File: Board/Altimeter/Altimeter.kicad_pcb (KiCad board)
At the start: 2 copper layers, 40 x 40 mm, 53 parts, among them J1 PWRIN, J2 STLink, J3 Micro_SD_Card_Det_Hirose_DM3AT, J4 GNSS, J5 RS485, J6 ReleaseSys, SW1 SW_RESET, U1 STM32L431RBTx, U2 LPS22HB_Module, U3 ST1480AxDR, Y1 FA238-20MHz, Y2 FC255-32.768kHz

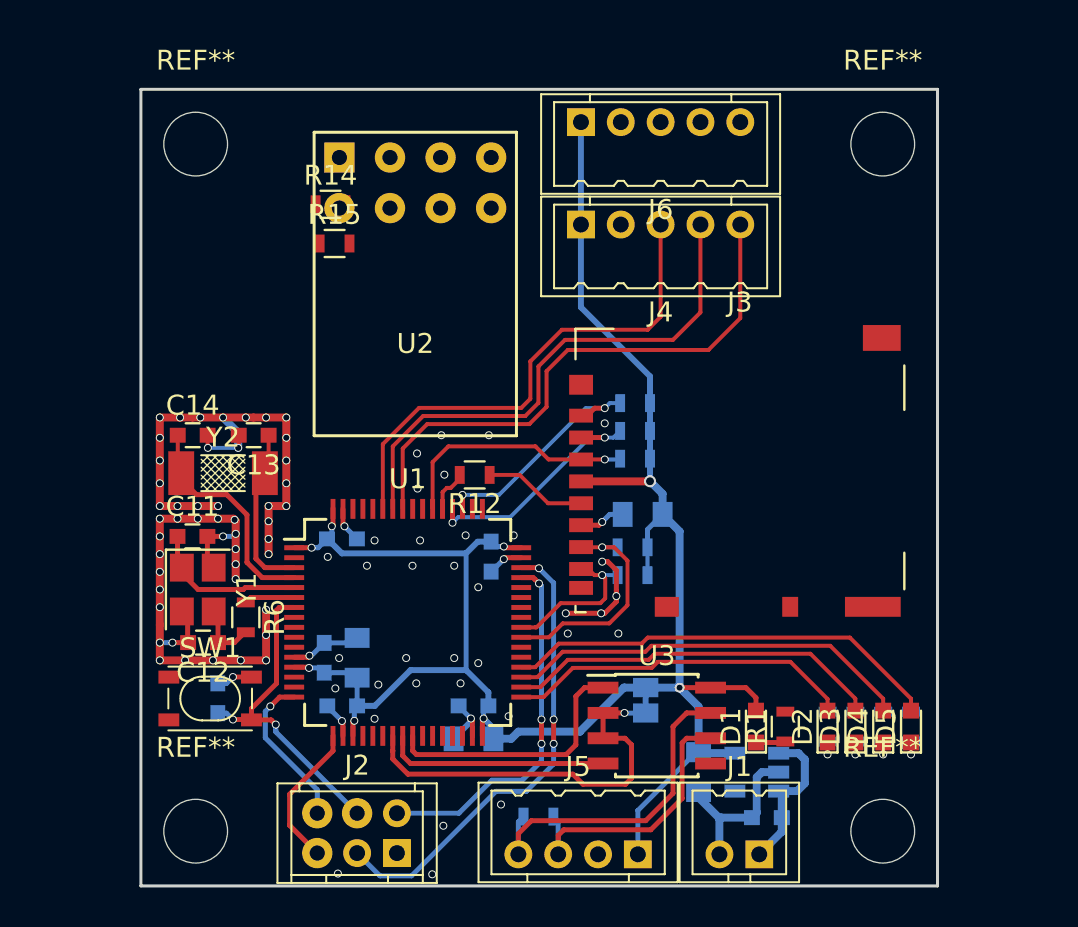
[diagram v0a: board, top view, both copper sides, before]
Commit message: almost complete (size:50x30) task: silk and via
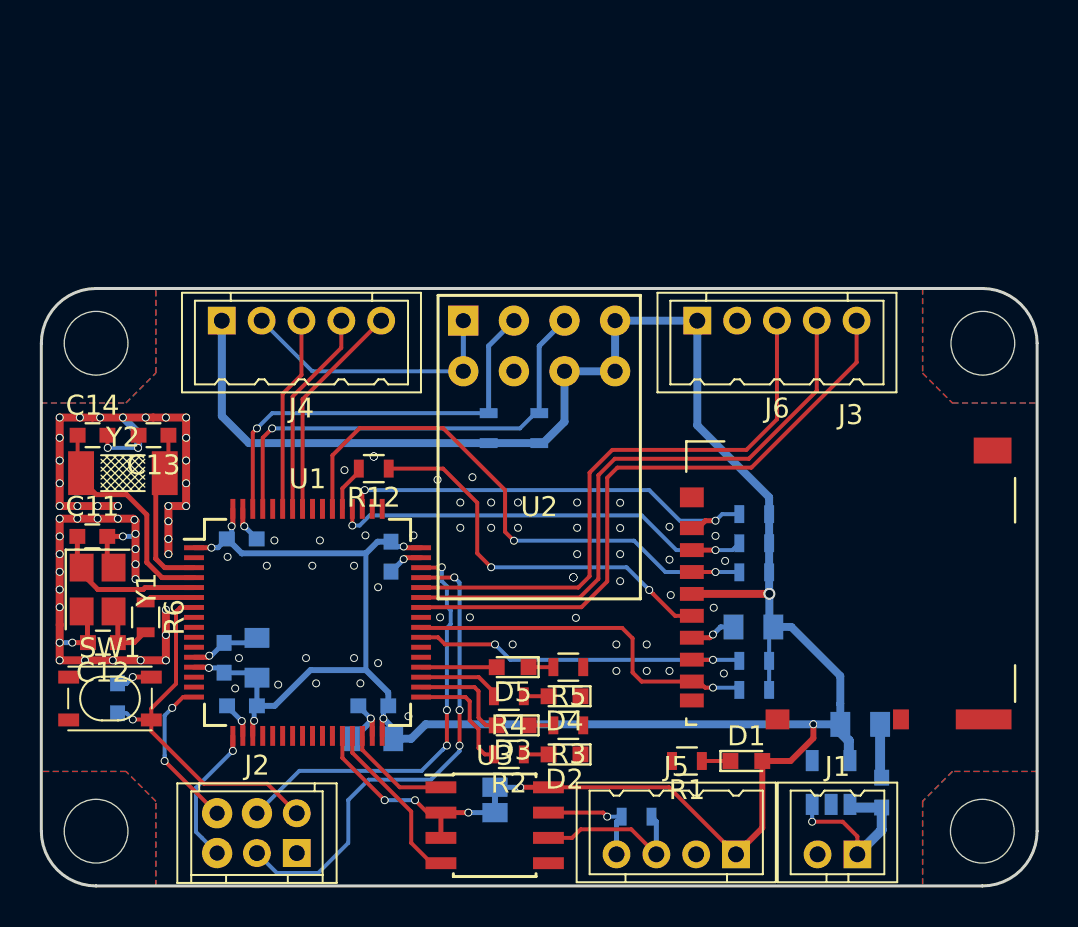
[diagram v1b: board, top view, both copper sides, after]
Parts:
- removed the REF** at (167.2, 62.8)
- removed the REF** at (167.2, 97.2)
- removed the REF** at (132.8, 97.2)
- added REF**: MountingHole_3.2mm_M3, Mounting_Holes:MountingHole_3.2mm_M3, F.Cu at (172.3, 72.8)
- added REF**: MountingHole_3.2mm_M3, Mounting_Holes:MountingHole_3.2mm_M3, F.Cu at (172.2, 97.2)
- added REF**: MountingHole_3.2mm_M3, Mounting_Holes:MountingHole_3.2mm_M3, F.Cu at (127.8, 97.2)
- R14, R15: moved to B.Cu
- R2, R3, R4, R5: moved to F.Cu
- moved D5 20.2 mm to (148.7, 89.0), turned to 180 degrees
- moved R4 18.9 mm to (148.5, 90.5), turned to 180 degrees
- moved J4 18.7 mm to (138.1, 71.6)
- moved R5 17.5 mm to (151.5, 89.0), turned to 180 degrees
- moved D3 17.2 mm to (148.7, 91.9), turned to 180 degrees
- moved D4 16.1 mm to (151.3, 90.5), turned to 180 degrees
- moved R2 16.1 mm to (148.5, 93.4), turned to 180 degrees
- moved R3 14.4 mm to (151.5, 91.9), turned to 180 degrees
- moved R15 13.8 mm to (150.0, 77.0), turned to 90 degrees
- moved R14 13.8 mm to (147.5, 77.0), turned to 90 degrees
- moved D2 13.3 mm to (151.3, 93.4), turned to 180 degrees
- moved J6 11.6 mm to (161.9, 71.6)
- moved REF** 11.2 mm to (127.8, 72.8)
- moved U2 10.3 mm to (150.0, 78.0)
- moved U3 9.56 mm to (147.8, 97.0)
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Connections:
- D2 pad 1: Net-(D2-Pad1) -> GND
- D2 pad 2: /LED_R -> Net-(D2-Pad2)
- D4 pad 1: Net-(D4-Pad1) -> GND
- D4 pad 2: /LED_G -> Net-(D4-Pad2)
- J2 pad 2: /SWDIO -> /RESET
- J2 pad 3: /SWCLK -> /SWDIO
- J2 pad 4: /RESET -> /SWCLK
- J6 pad 3: (no net) -> /TRIGGER
- J6 pad 4: (no net) -> /BUZZER
- J6 pad 5: (no net) -> /FLIGHTPIN
- R2 pad 1: GND -> Net-(D2-Pad2)
- R2 pad 2: Net-(D2-Pad1) -> /LED_R
- R4 pad 1: GND -> Net-(D4-Pad2)
- R4 pad 2: Net-(D4-Pad1) -> /LED_G
- U1 pad 23: /RS485_EN -> (no net)
- U1 pad 24: /RS485_TX -> (no net)
- U1 pad 25: /RS485_RX -> (no net)
- U1 pad 28: (no net) -> /RS485_EN
- U1 pad 29: (no net) -> /RS485_TX
- U1 pad 30: (no net) -> /RS485_RX
- U1 pad 42: (no net) -> /FLIGHTPIN
- U1 pad 43: (no net) -> /BUZZER
- U1 pad 44: (no net) -> /TRIGGER
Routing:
- net +3V3: track 101.7 -> 150.2 mm, vias 8 -> 9
- net /FLIGHTPIN: track 0.00 -> 32.1 mm
- net /BUZZER: track 0.00 -> 30.7 mm
- net /TRIGGER: track 0.00 -> 29.4 mm
- net /I2C1_SCL: track 0.00 -> 23.1 mm, vias 0 -> 1
- net /I2C1_SDA: track 0.00 -> 21.3 mm, vias 0 -> 1
- net /LED_B: track 22.1 -> 3.80 mm
- net /GNSS_1PPS: track 28.4 -> 11.1 mm
- net /SD_CMD: track 12.4 -> 29.1 mm, vias 1 -> 2
- net /GNSS_TX: track 26.9 -> 10.5 mm
- net /LED_G: track 20.5 -> 4.17 mm
- net /GNSS_RX: track 25.6 -> 9.84 mm
- net Net-(J3-Pad5): track 5.18 -> 19.8 mm, vias 0 -> 2
- net /LED_Y: track 19.0 -> 5.38 mm
- net /LED_R: track 17.5 -> 5.97 mm
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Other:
- board size 40 x 40 mm -> 50 x 30 mm
